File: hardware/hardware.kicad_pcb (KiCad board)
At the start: 2 copper layers, 127 x 88.9 mm, 55 parts, among them J1 USB_C_Receptacle_USB2.0, J2 AudioPlug4, J3 USB_C_Receptacle_USB2.0, J4 AudioPlug4, SW1 SW_Push, SW2 SW_Push, SW3 SW_Push, SW4 SW_Push, SW5 SW_Push, SW6 SW_Push, SW7 SW_Push, SW8 SW_Push, U1 ProMicro, U3 ATMEGA32U4, Y1 16MHz

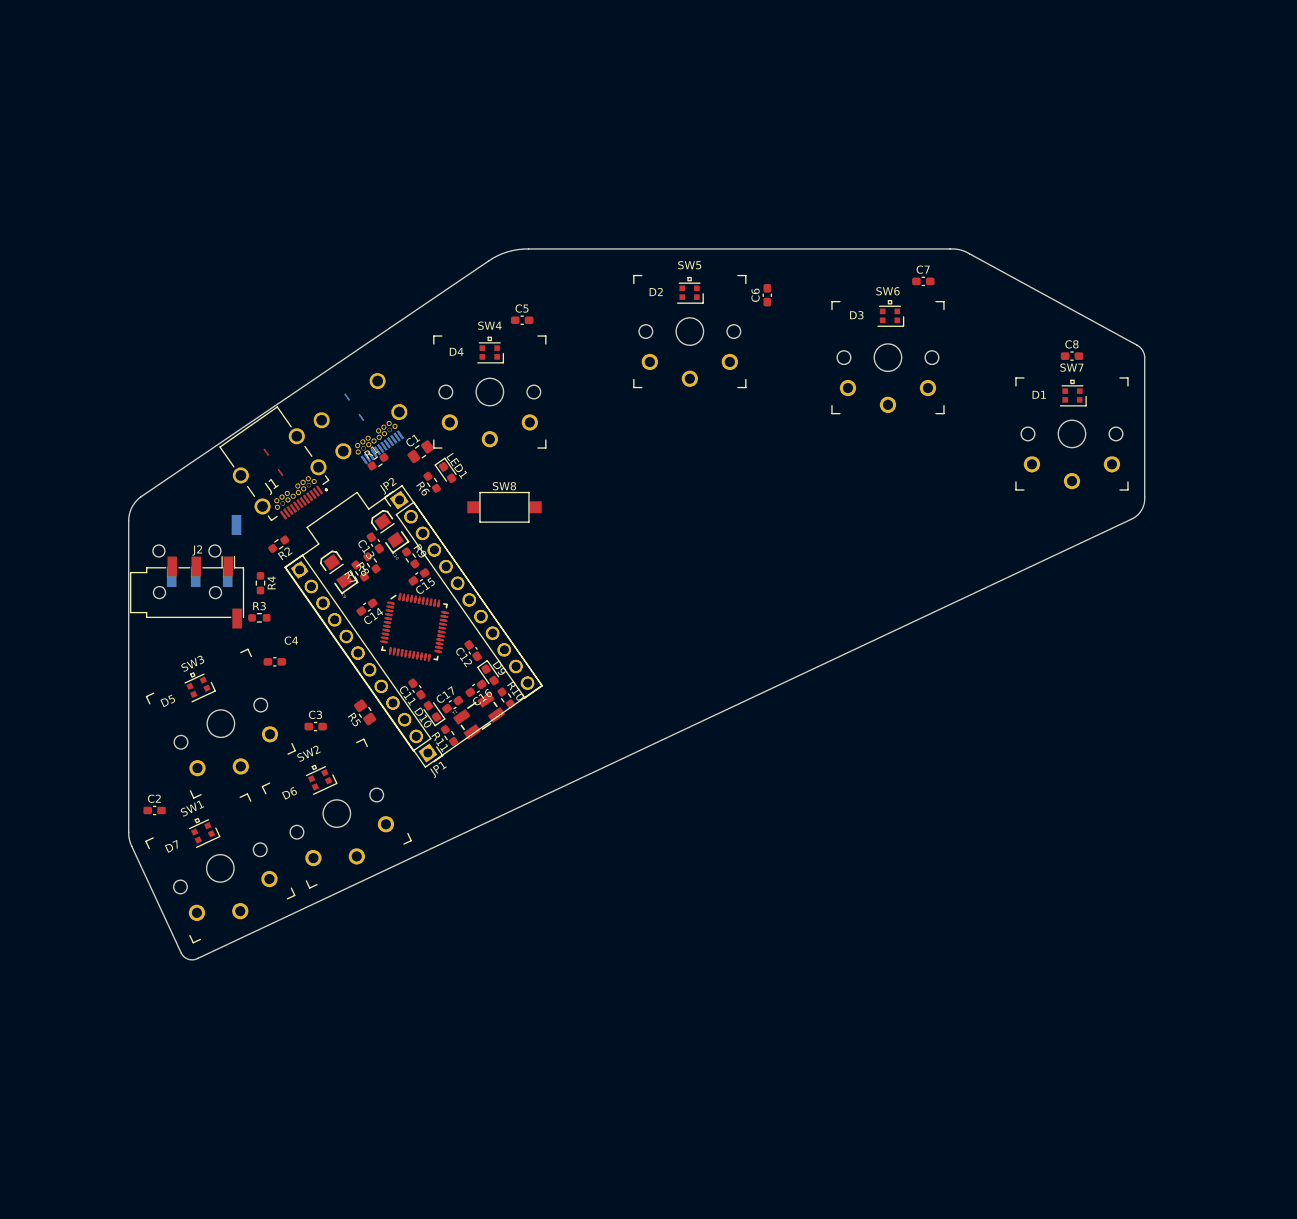
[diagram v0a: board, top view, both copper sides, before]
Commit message: start routing
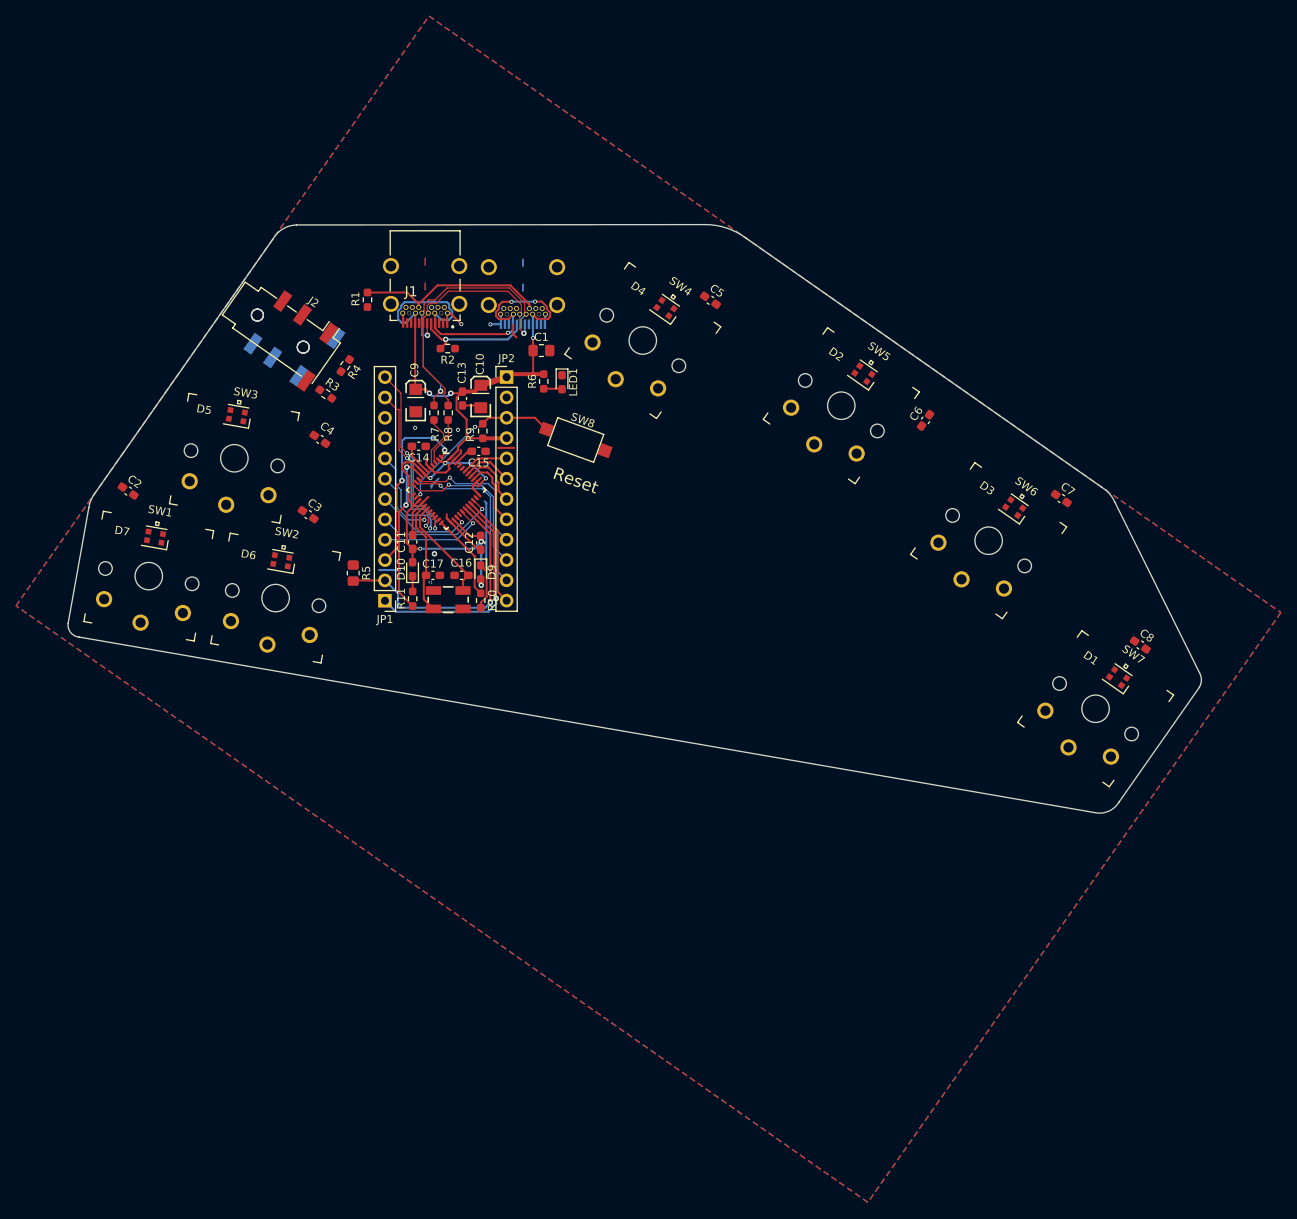
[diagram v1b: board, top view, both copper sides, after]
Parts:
- removed U1: ProMicro, Library:ProMicro
- moved C2 40.1 mm to (-0.07, 30.3), turned to -35 degrees
- moved SW1 37.6 mm to (2.51, 40.9), turned to -10 degrees
- moved D7 37.4 mm to (3.29, 36.0), turned to -10 degrees
- moved C8 37.1 mm to (126.4, 49.5), turned to -35 degrees
- moved D1 35.7 mm to (123.7, 53.6), turned to -35 degrees
- moved SW7 34.5 mm to (120.9, 57.5), turned to -35 degrees
- moved D5 34.3 mm to (13.5, 20.8), turned to -10 degrees
- moved J2 33.9 mm to (20.0, 11.0), turned to -35 degrees
- moved SW3 33.2 mm to (13.2, 26.2), turned to -10 degrees
- moved R2 32.3 mm to (39.9, 12.4), turned to 180 degrees
- moved C7 32.2 mm to (116.6, 31.2), turned to -35 degrees
- moved J1 29.9 mm to (37.1, 3.78), turned to 180 degrees
- moved R4 29.2 mm to (27.1, 14.6), turned to -125 degrees
- moved R3 29.2 mm to (24.6, 18.1), turned to -35 degrees
- moved J4 29.1 mm to (20.0, 11.0), turned to -35 degrees
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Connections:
- J1 pad B5: Net-(J1-PadB5) -> Net-(J3-PadB5)
- J2 pad T: BTN1 -> SCK
- J3 pad A5: GND -> Net-(J1-PadA5)
- J3 pad B5: GND -> Net-(J3-PadB5)
- J4 pad T: BTN1 -> SCK
- JP1 pad 7: BTN1 -> SCK
- R1 pad 1: Net-(J1-PadA5) -> Net-(J3-PadB5)
- R2 pad 1: Net-(J1-PadB5) -> GND
- R2 pad 2: GND -> Net-(J1-PadA5)
- R4 pad 1: BTN1 -> SCK
- R5 pad 1: Net-(R5-Pad1) -> GND
- R5 pad 2: GND -> /Pro Micro/D8
- SW8 pad 1: Net-(U1-Pad22) -> /Pro Micro/RESET
- U3 pad 18: BTN1 -> SCK
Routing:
- net +5V: track 0.00 -> 144.9 mm, vias 0 -> 12
- net GND: track 0.00 -> 50.6 mm, vias 0 -> 5
- net USB_D+: track 0.00 -> 33.4 mm, vias 0 -> 2
- net /Pro Micro/D8: track 0.00 -> 32.8 mm, vias 0 -> 1
- net USB_D-: track 0.00 -> 32.6 mm, vias 0 -> 1
- net LED_IN: track 0.00 -> 28.6 mm, vias 0 -> 1
- net Net-(J3-PadB5): track 0.00 -> 23.7 mm
- net /Pro Micro/TXO: track 0.00 -> 23.5 mm, vias 0 -> 2
- net BTN4: track 0.00 -> 23.1 mm, vias 0 -> 2
- net /Pro Micro/RESET: track 0.00 -> 22.0 mm, vias 0 -> 2
- net /Pro Micro/RXI: track 0.00 -> 21.6 mm, vias 0 -> 2
- net BTN2: track 0.00 -> 21.3 mm, vias 0 -> 1
- net /Pro Micro/D14: track 0.00 -> 20.8 mm, vias 0 -> 2
- net BTN3: track 0.00 -> 19.8 mm, vias 0 -> 1
- net BTN1: track 0.00 -> 17.3 mm, vias 0 -> 1
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- added copper zone on B.Cu, net GND
- added copper zone on F.Cu, net GND
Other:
- board size 127 x 88.9 mm -> 141.7 x 73.6 mm
- board text added: "Reset"
